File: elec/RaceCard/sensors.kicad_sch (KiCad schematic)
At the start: 25 parts, among them U10 4ch_Slider, U2 IQS7222A001QFR, U7 BTN1, U8 BTN2, U9 BTN3

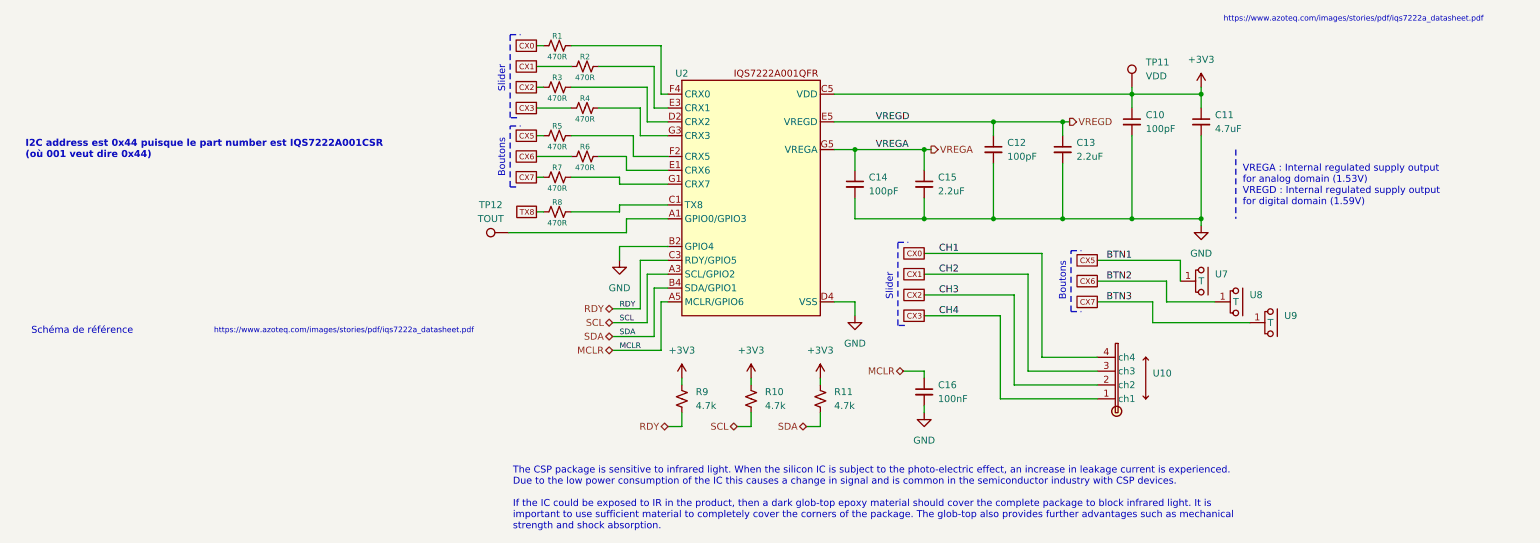
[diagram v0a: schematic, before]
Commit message: Cleanup
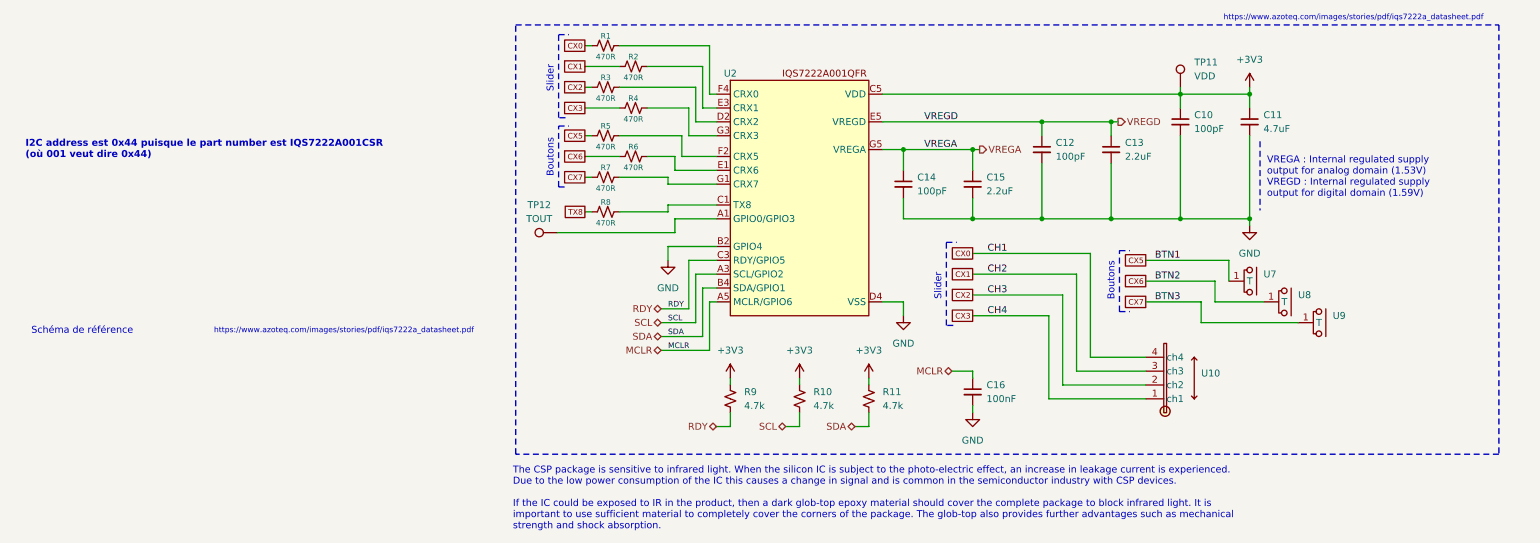
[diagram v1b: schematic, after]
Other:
- moved on the sheet: C10, C11, C12, C13, C14, C15, C16, R1, R10, R11, R2, R3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
